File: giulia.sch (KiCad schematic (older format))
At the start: 1 part

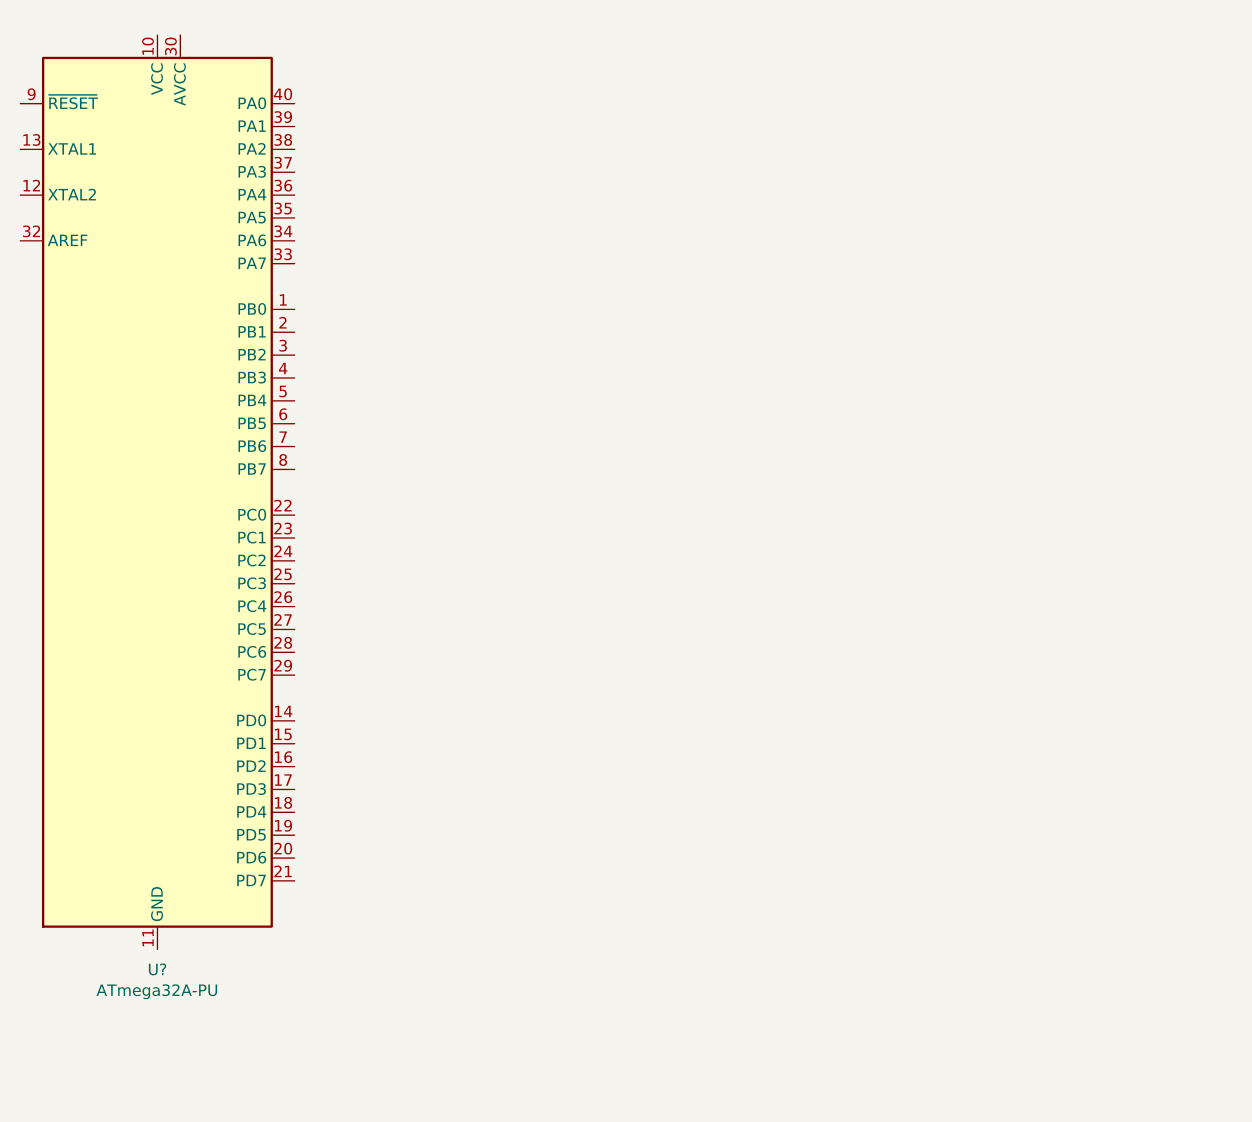
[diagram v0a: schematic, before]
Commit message: basic MCU wiring
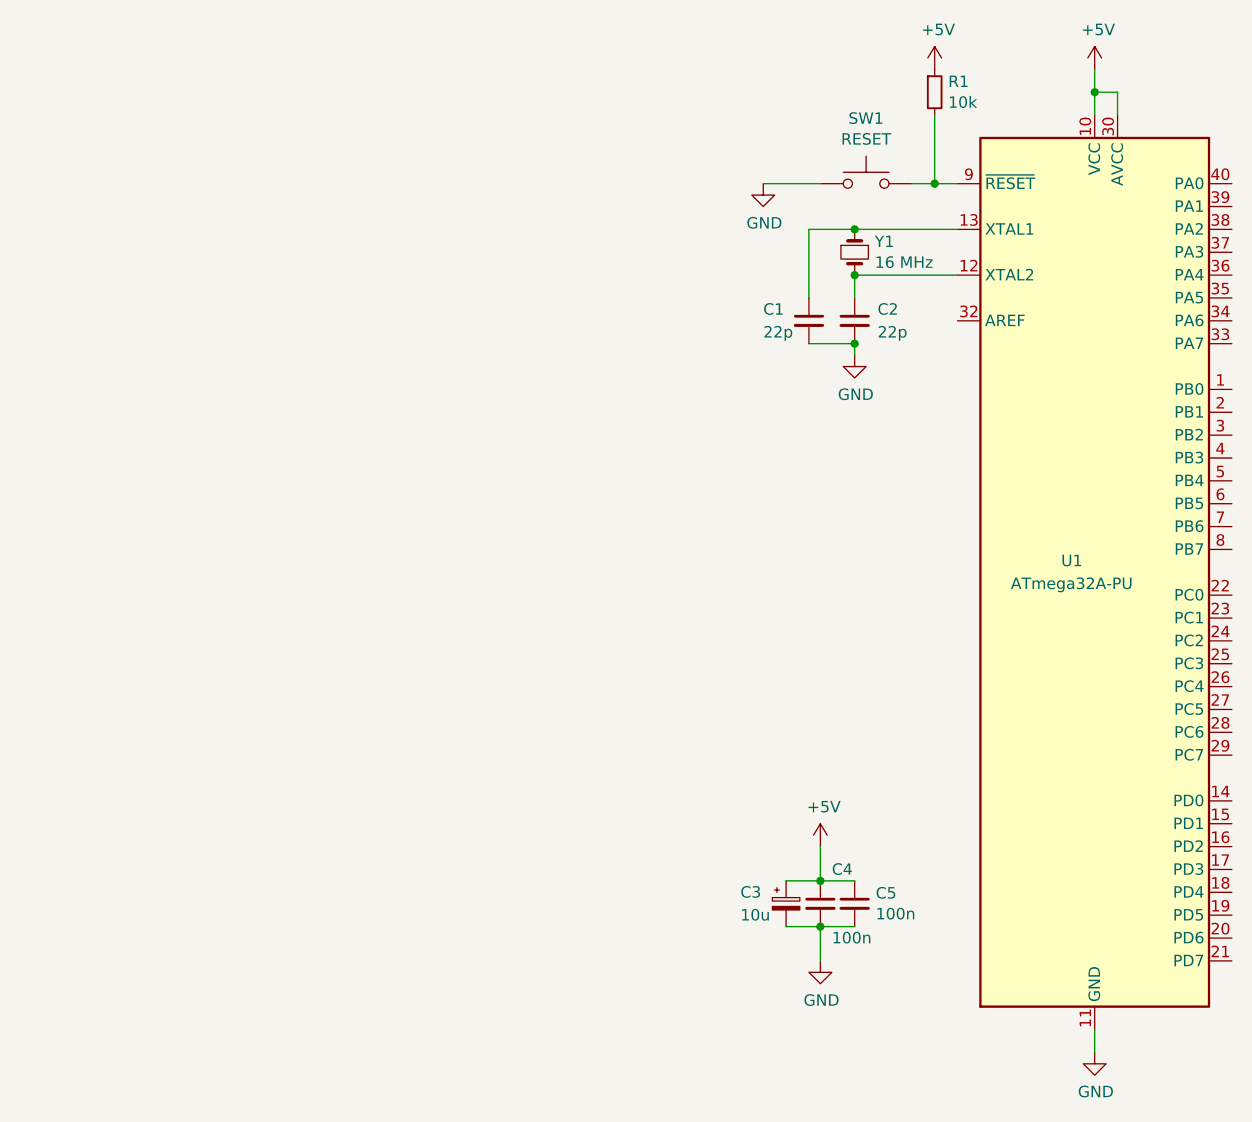
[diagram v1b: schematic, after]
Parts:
- added C1, C2: 22p, symbol Device:C_Small
- added C3: 10u, symbol Device:CP_Small
- added C4, C5: 100n, symbol Device:C_Small
- added R1: 10k, symbol Device:R_Small
- added SW1: RESET, symbol Switch:SW_Push
- added Y1: 16 MHz, symbol Device:Crystal_Small
- gave numbers to parts that had none: 1
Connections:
- net +5V: now reaches U1.10 (VCC)
- net +5V: now also U1.30 (AVCC), C3.1, C4.1, C5.1, R1.1
- net GND: now reaches U1.11 (GND), U1.31 (GND)
- net GND: now also C1.2, C2.2, C3.2, C4.2, C5.2, SW1.1
- net at U1.12 (XTAL2): now also C2.1, Y1.2
- net at U1.13 (XTAL1): now also C1.1, Y1.1
- net at U1.9 (~RESET): now also R1.2, SW1.2
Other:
- moved on the sheet: U1
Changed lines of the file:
@@
 $EndDescr
 $Comp
-L MCU_Microchip_ATmega:ATmega32A-PU U?
+L MCU_Microchip_ATmega:ATmega32A-PU U1
 U 1 1 6106E53B
-P 1500 3400
-F 0 "U?" H 1500 1311 50  0000 C CNN
-F 1 "ATmega32A-PU" H 1500 1220 50  0000 C CNN
-F 2 "Package_DIP:DIP-40_W15.24mm" H 1500 3400 50  0001 C CIN
-F 3 "http://ww1.microchip.com/downloads/en/DeviceDoc/atmel-8155-8-bit-microcontroller-avr-atmega32a_datasheet.pdf" H 1500 3400 50  0001 C CNN
-	1    1500 3400
-	1    0    0    -1
-$EndComp
+P 5600 3750
+F 0 "U1" H 5500 3800 50  0000 C CNN
+F 1 "ATmega32A-PU" H 5500 3700 50  0000 C CNN
+F 2 "Package_DIP:DIP-40_W15.24mm" H 5600 3750 50  0001 C CIN
+F 3 "http://ww1.microchip.com/downloads/en/DeviceDoc/atmel-8155-8-bit-microcontroller-avr-atmega32a_datasheet.pdf" H 5600 3750 50  0001 C CNN
+	1    5600 3750
+	1    0    0    -1
+$EndComp
+$Comp
+L power:+5V #PWR?
+U 1 1 6107440A
+P 5600 1550
+F 0 "#PWR?" H 5600 1400 50  0001 C CNN
+F 1 "+5V" H 5615 1723 50  0000 C CNN
+F 2 "" H 5600 1550 50  0001 C CNN
+F 3 "" H 5600 1550 50  0001 C CNN
+	1    5600 1550
+	1    0    0    -1
+$EndComp
+Wire Wire Line
+	5600 1550 5600 1650
+Wire Wire Line
+	5700 1750 5700 1650
+Wire Wire Line
+	5700 1650 5600 1650
+Connection ~ 5600 1650
+Wire Wire Line
+	5600 1650 5600 1750
+$Comp
+L power:GND #PWR?
+U 1 1 610754C4
+P 5600 5850
+F 0 "#PWR?" H 5600 5600 50  0001 C CNN
+F 1 "GND" H 5605 5677 50  0000 C CNN
+F 2 "" H 5600 5850 50  0001 C CNN
+F 3 "" H 5600 5850 50  0001 C CNN
+	1    5600 5850
+	1    0    0    -1
+$EndComp
+$Comp
+L Device:C_Small C2
+U 1 1 6108361C
+P 4550 2650
+F 0 "C2" H 4650 2700 50  0000 L CNN
+F 1 "22p" H 4650 2600 50  0000 L CNN
+F 2 "" H 4550 2650 50  0001 C CNN
+F 3 "~" H 4550 2650 50  0001 C CNN
+	1    4550 2650
+	1    0    0    -1
+$EndComp
+$Comp
+L Device:C_Small C1
+U 1 1 61085D6B
+P 4350 2650
+F 0 "C1" H 4150 2700 50  0000 L CNN
+F 1 "22p" H 4150 2600 50  0000 L CNN
+F 2 "" H 4350 2650 50  0001 C CNN
+F 3 "~" H 4350 2650 50  0001 C CNN
+	1    4350 2650
+	1    0    0    -1
+$EndComp
+$Comp
+L power:GND #PWR?
+U 1 1 610873C2
+P 4550 2800
+F 0 "#PWR?" H 4550 2550 50  0001 C CNN
+F 1 "GND" H 4555 2627 50  0000 C CNN
+F 2 "" H 4550 2800 50  0001 C CNN
+F 3 "" H 4550 2800 50  0001 C CNN
+	1    4550 2800
+	1    0    0    -1
+$EndComp
+$Comp
+L Device:Crystal_Small Y1
+U 1 1 610C25E9
+P 4550 2350
+F 0 "Y1" V 4504 2438 50  0000 L CNN
+F 1 "16 MHz" V 4595 2438 50  0000 L CNN
+F 2 "" H 4550 2350 50  0001 C CNN
+F 3 "~" H 4550 2350 50  0001 C CNN
+	1    4550 2350
+	0    1    1    0
+$EndComp
+Wire Wire Line
+	5000 2250 4550 2250
+Wire Wire Line
+	5000 2450 4550 2450
+Wire Wire Line
+	4550 2250 4350 2250
+Wire Wire Line
+	4350 2250 4350 2550
+Connection ~ 4550 2250
+Wire Wire Line
+	4550 2550 4550 2450
+Connection ~ 4550 2450
+Wire Wire Line
+	4550 2750 4550 2800
+Wire Wire Line
+	4350 2750 4550 2750
+Connection ~ 4550 2750
+Wire Wire Line
+	5600 5850 5600 5750
+$Comp
+L power:+5V #PWR?
+U 1 1 610DE068
+P 4400 4950
+F 0 "#PWR?" H 4400 4800 50  0001 C CNN
+F 1 "+5V" H 4415 5123 50  0000 C CNN
+F 2 "" H 4400 4950 50  0001 C CNN
+F 3 "" H 4400 4950 50  0001 C CNN
+	1    4400 4950
+	1    0    0    -1
+$EndComp
+$Comp
+L Device:C_Small C4
+U 1 1 610DF006
+P 4400 5200
+F 0 "C4" H 4450 5350 50  0000 L CNN
+F 1 "100n" H 4450 5050 50  0000 L CNN
+F 2 "" H 4400 5200 50  0001 C CNN
+F 3 "~" H 4400 5200 50  0001 C CNN
+	1    4400 5200
+	1    0    0    -1
+$EndComp
+$Comp
+L Device:C_Small C5
+U 1 1 610E006A
+P 4550 5200
+F 0 "C5" H 4642 5246 50  0000 L CNN
+F 1 "100n" H 4642 5155 50  0000 L CNN
+F 2 "" H 4550 5200 50  0001 C CNN
+F 3 "~" H 4550 5200 50  0001 C CNN
+	1    4550 5200
+	1    0    0    -1
+$EndComp
+Wire Wire Line
+	4550 5100 4400 5100
+Connection ~ 4400 5100
+Wire Wire Line
+	4550 5300 4400 5300
+$Comp
+L Device:CP_Small C3
+U 1 1 610E14C2
+P 4250 5200
+F 0 "C3" H 4050 5250 50  0000 L CNN
+F 1 "10u" H 4050 5150 50  0000 L CNN
+F 2 "" H 4250 5200 50  0001 C CNN
+F 3 "~" H 4250 5200 50  0001 C CNN
+	1    4250 5200
+	1    0    0    -1
+$EndComp
+Wire Wire Line
+	4250 5100 4400 5100
+Wire Wire Line
+	4250 5300 4400 5300
+Connection ~ 4400 5300
+$Comp
+L power:GND #PWR?
+U 1 1 610E3173
+P 4400 5450
+F 0 "#PWR?" H 4400 5200 50  0001 C CNN
+F 1 "GND" H 4405 5277 50  0000 C CNN
+F 2 "" H 4400 5450 50  0001 C CNN
+F 3 "" H 4400 5450 50  0001 C CNN
+	1    4400 5450
+	1    0    0    -1
+$EndComp
+Wire Wire Line
+	4400 5450 4400 5300
+Wire Wire Line
+	4400 5100 4400 4950
+$Comp
+L Switch:SW_Push SW1
+U 1 1 610E88B8
+P 4600 2050
+F 0 "SW1" H 4600 2335 50  0000 C CNN
+F 1 "RESET" H 4600 2244 50  0000 C CNN
+F 2 "" H 4600 2250 50  0001 C CNN
+F 3 "~" H 4600 2250 50  0001 C CNN
+	1    4600 2050
+	1    0    0    -1
+$EndComp
+$Comp
+L power:GND #PWR?
+U 1 1 610E92D6
+P 4150 2050
+F 0 "#PWR?" H 4150 1800 50  0001 C CNN
+F 1 "GND" H 4155 1877 50  0000 C CNN
+F 2 "" H 4150 2050 50  0001 C CNN
+F 3 "" H 4150 2050 50  0001 C CNN
+	1    4150 2050
+	1    0    0    -1
+$EndComp
+Wire Wire Line
+	4150 2050 4400 2050
+$Comp
+L Device:R_Small R1
+U 1 1 610EA94C
+P 4900 1650
+F 0 "R1" H 4959 1696 50  0000 L CNN
+F 1 "10k" H 4959 1605 50  0000 L CNN
+F 2 "" H 4900 1650 50  0001 C CNN
+F 3 "~" H 4900 1650 50  0001 C CNN
+	1    4900 1650
+	1    0    0    -1
+$EndComp
+$Comp
+L power:+5V #PWR?
+U 1 1 610EB5A6
+P 4900 1550
+F 0 "#PWR?" H 4900 1400 50  0001 C CNN
+F 1 "+5V" H 4915 1723 50  0000 C CNN
+F 2 "" H 4900 1550 50  0001 C CNN
+F 3 "" H 4900 1550 50  0001 C CNN
+	1    4900 1550
+	1    0    0    -1
+$EndComp
+Wire Wire Line
+	4800 2050 4900 2050
+Wire Wire Line
+	4900 1750 4900 2050
+Connection ~ 4900 2050
+Wire Wire Line
+	4900 2050 5000 2050
 $EndSCHEMATC
